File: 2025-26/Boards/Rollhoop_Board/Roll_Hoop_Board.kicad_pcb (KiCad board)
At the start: 2 copper layers, 106.7 x 32 mm, 24 parts, among them J1 DTM13-12PA, J2 DTM13-12PA, Q1 AO3401A, Q2 AO3400A, Q3 AO3400A, U1 AMS1117-3.3, U2 SN65HVD230, U3 STM32C011F4Px

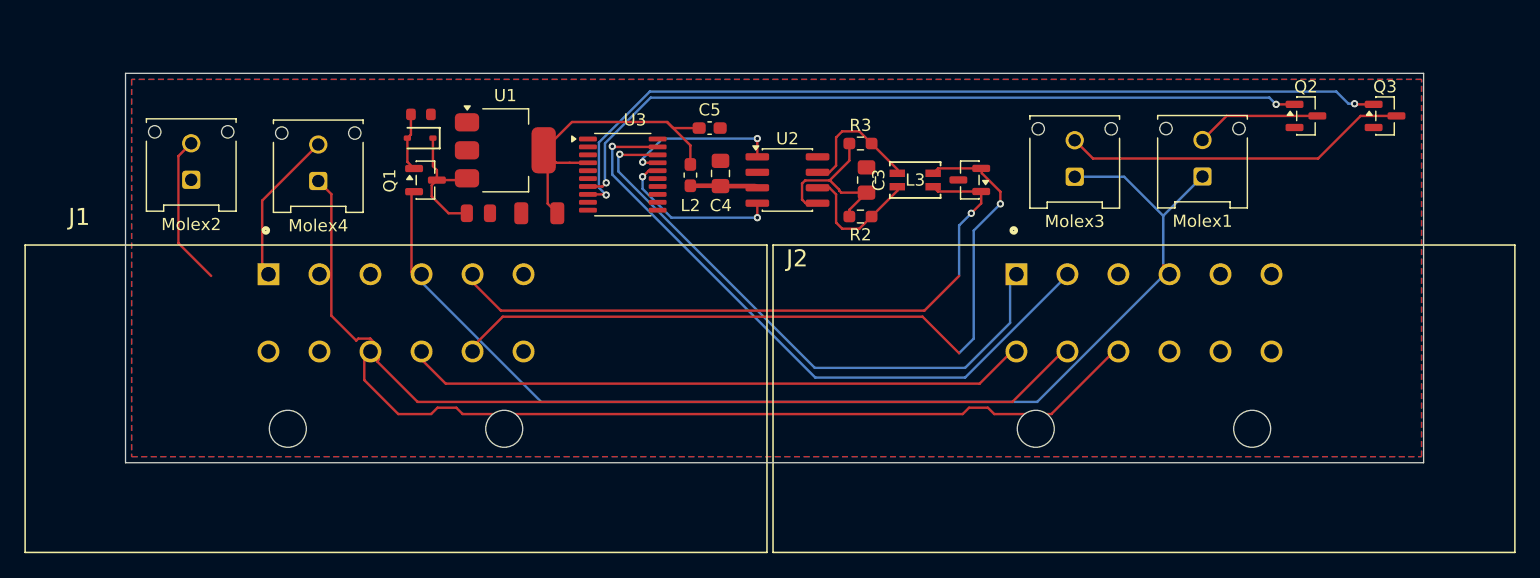
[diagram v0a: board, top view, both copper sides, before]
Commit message: Rollhoop edits
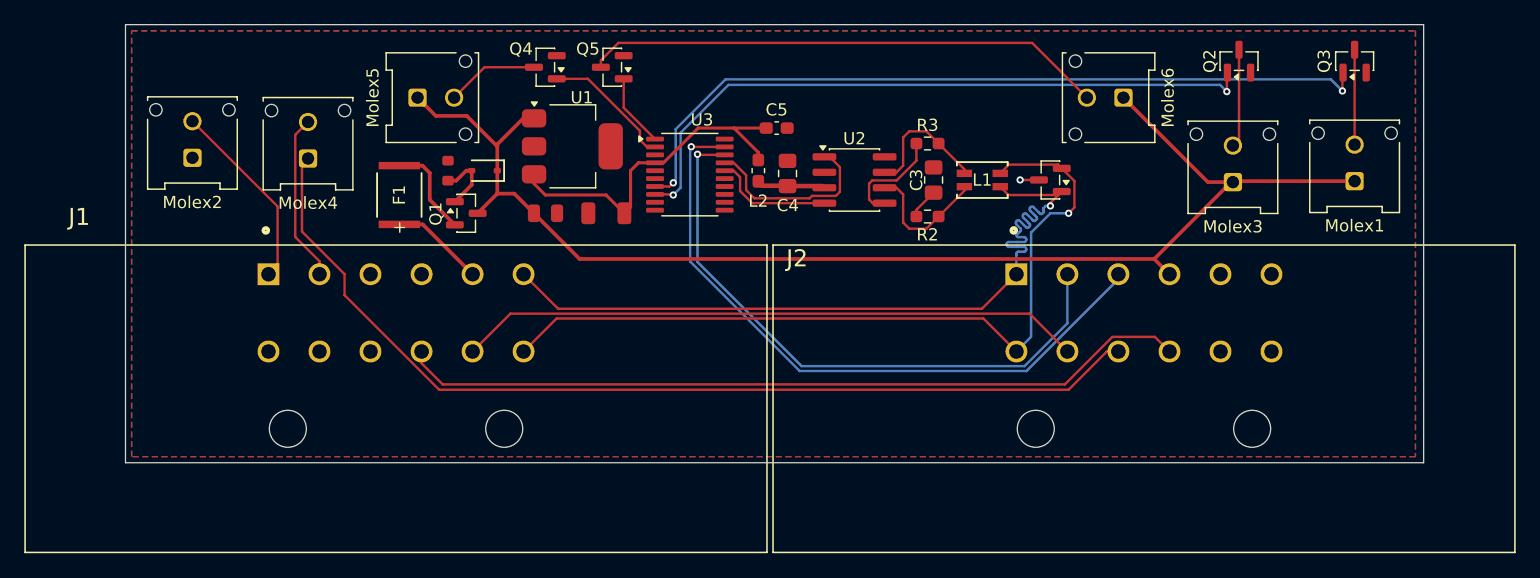
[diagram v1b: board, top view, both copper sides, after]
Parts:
- added F1: MINISMDC020F-2, MINISMDC020F-2:FUS_MINISMDC020F_TYCO_TYC, F.Cu at (138.5, 39.0)
- added Molex5: 043045-0212, Connector_Molex:Molex_Micro-Fit_3.0_43045-0212_2x01_P3.00mm_Vertical, F.Cu at (140.0, 31.0)
- added Molex6: 043045-0212, Connector_Molex:Molex_Micro-Fit_3.0_43045-0212_2x01_P3.00mm_Vertical, F.Cu at (198.0, 31.0)
- added Q4: AO3400A, Package_TO_SOT_SMD:SOT-23, F.Cu at (150.5, 28.5)
- added Q5: AO3400A, Package_TO_SOT_SMD:SOT-23, F.Cu at (156.0, 28.5)
- U1: value AMS1117-3.3 -> UA78M33QDCYRQ1
- moved Molex3 13.0 mm to (207.0, 37.9)
- moved Molex1 12.5 mm to (217.0, 37.9)
- moved Q2 7.11 mm to (207.5, 28.0), turned to 90 degrees
- moved D2 6.62 mm to (192.0, 37.8)
- moved D1 5.93 mm to (145.5, 37.0)
- moved L2 5.59 mm to (168.0, 37.0)
- moved U1 5.52 mm to (152.7, 35.0)
- moved C1 5.51 mm to (150.5, 40.5)
- moved C2 5.51 mm to (155.5, 40.5)
- moved C5 5.51 mm to (169.5, 33.5)
- moved C3 5.51 mm to (182.4, 37.8)
- moved C4 5.51 mm to (170.4, 37.2)
- moved L1 5.51 mm to (186.4, 37.8)
- moved R2 5.51 mm to (181.9, 40.8)
- moved R3 5.51 mm to (181.9, 34.8)
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- renumbered L3 to L1
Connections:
- J2 pad 4: unconnected-(J2-Pad4) -> DSH_PWR
- J2 pad 5: DSH_PWR -> unconnected-(J2-Pad5)
- Molex1 pad 1: +12V -> Net-(Q1-D)
- Molex3 pad 1: +12V -> Net-(Q1-D)
- Q2 pad 1: Green_LED -> Red_LED
- Q2 pad 3: Green_Out -> Red_Out
- Q3 pad 1: Red_LED -> Green_LED
- Q3 pad 3: Red_Out -> Green_Out
- U1 pad 1: GND -> Net-(Q1-D)
- U1 pad 2: RLH_3.3V -> GND
- U1 pad 3: Net-(Q1-D) -> RLH_3.3V
- U3 pad 1: unconnected-(U3-PB7-Pad1) -> Buzzer2
- U3 pad 2: unconnected-(U3-PC14-Pad2) -> Buzzer1
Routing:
- net DSH_PWR: track 131.9 -> 7.77 mm
- net Net-(Q1-D): track 11.1 -> 107.4 mm
- net DSH_CAN_L: track 12.1 -> 66.4 mm
- net DSH_CAN_H: track 21.4 -> 66.6 mm
- net Buzzer2_Out: track 0.00 -> 43.0 mm
- net DSH_CAN_S: track 93.9 -> 51.5 mm
- net Red_Out: track 28.5 -> 8.08 mm
- net Red_LED: track 71.9 -> 55.2 mm
- net Buzzer1: track 0.00 -> 10.8 mm
- net Net-(Q1-S): track 0.00 -> 7.87 mm
- net Buzzer1_Out: track 0.00 -> 7.60 mm
- net (no net): track 7.14 -> 0.00 mm
- net Buzzer2: track 0.00 -> 6.02 mm
- net RX: track 14.0 -> 9.97 mm, vias 2 -> 0
- net DSH_SDC_IN: track 77.1 -> 81.0 mm
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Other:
- board size 106.7 x 32 mm -> 106.7 x 36 mm
